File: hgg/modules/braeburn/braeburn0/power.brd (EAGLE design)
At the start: 104.4 x 75 mm, 69 parts, among them IC1 LM324D, IC4 ATMEGA48/88/168-AU, IC5 LTC485S, Q1 20Mhz

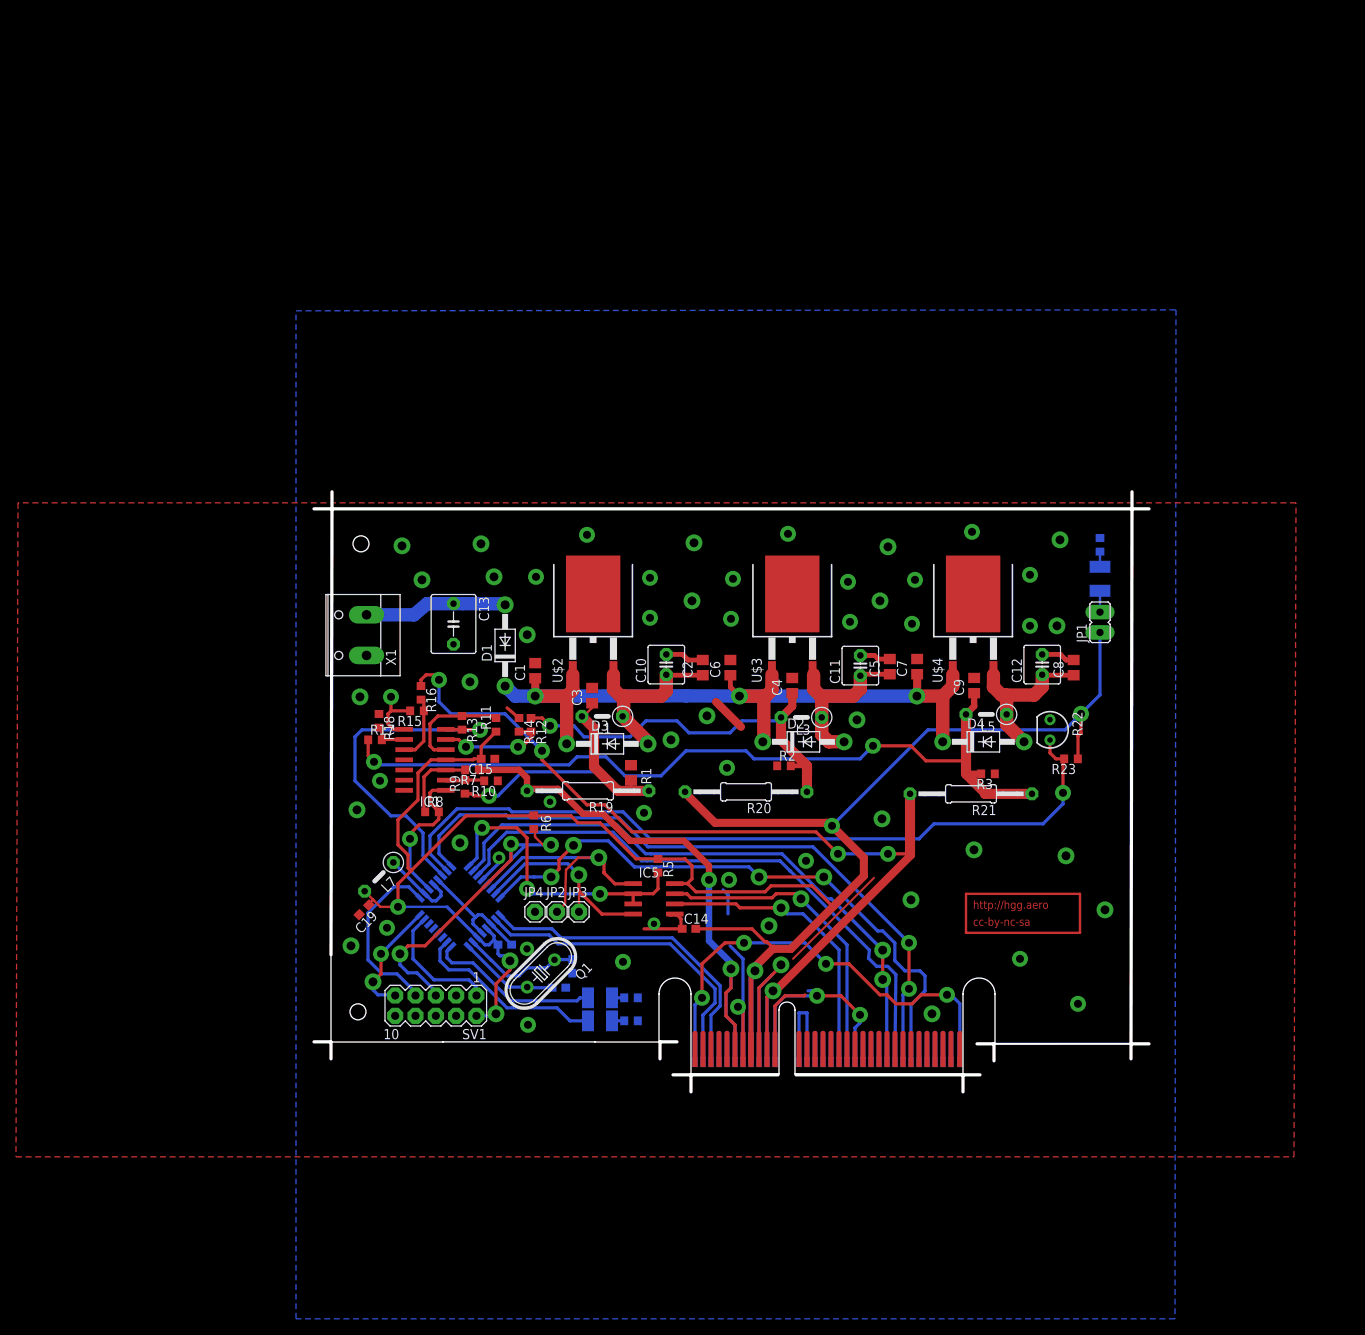
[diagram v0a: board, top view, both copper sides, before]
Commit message: updates versoin of braeburn
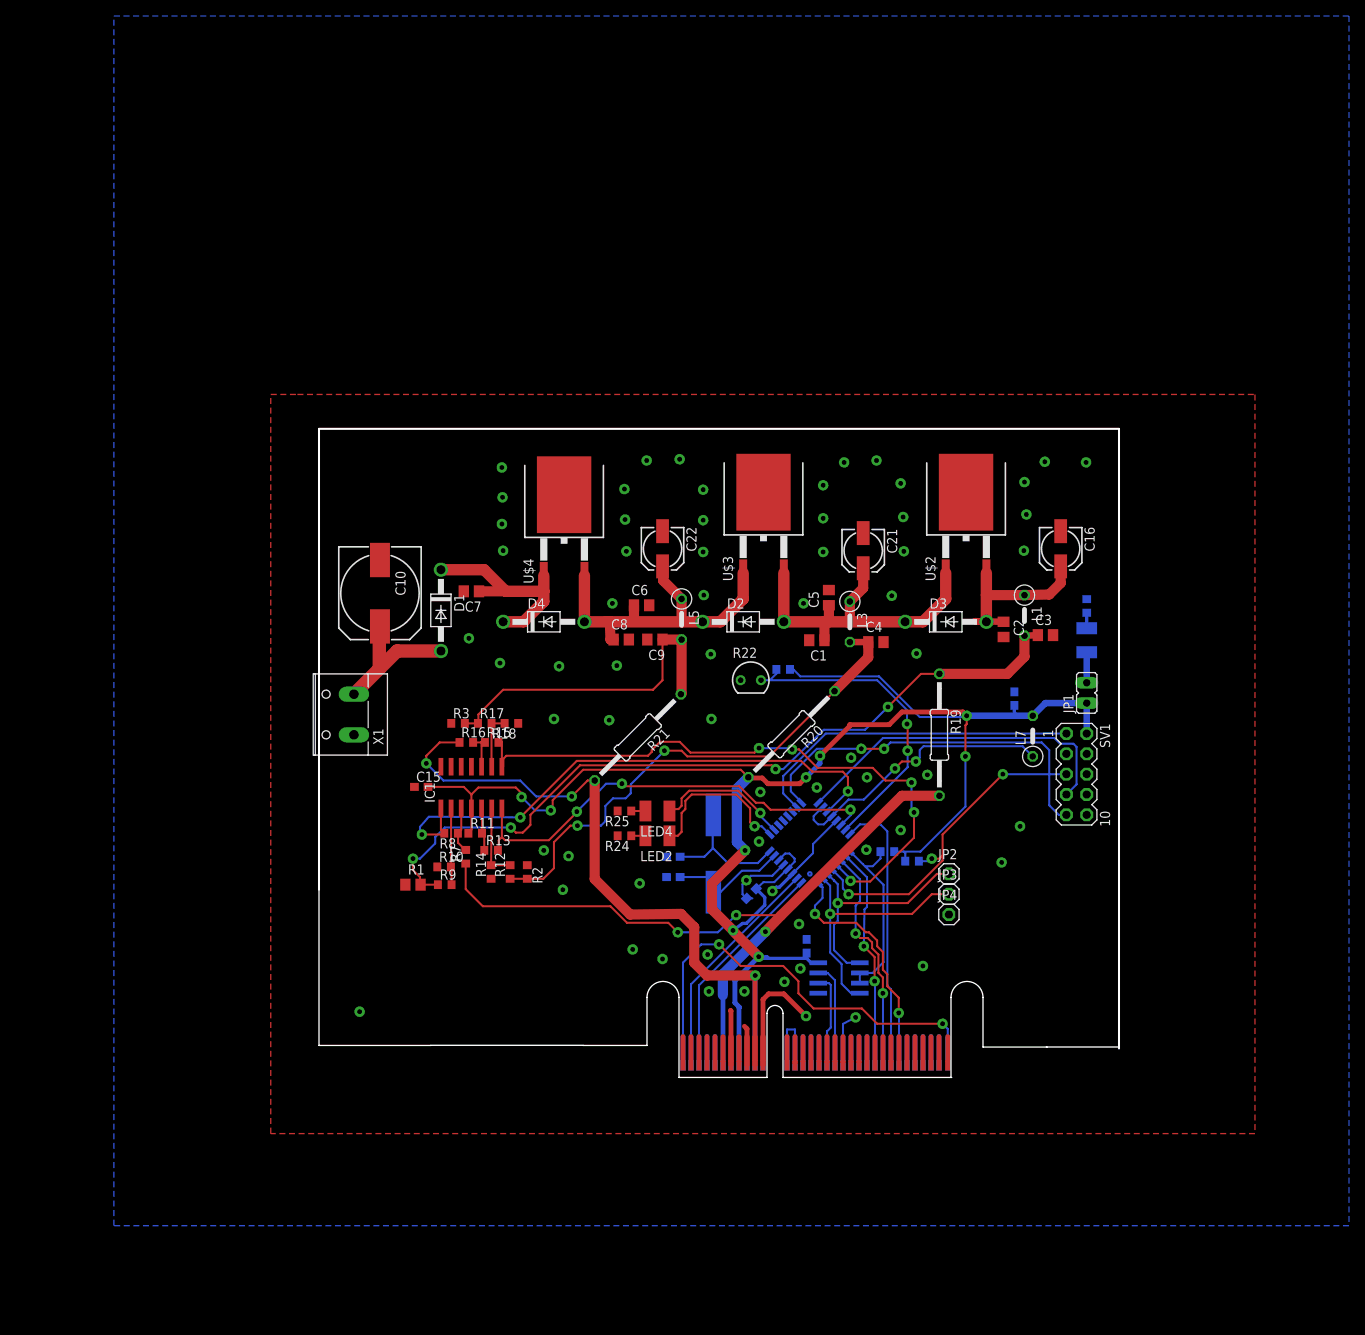
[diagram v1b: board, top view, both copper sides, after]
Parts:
- removed C11, C12: (no value), rcl:C025-050X050
- removed C13: 2000u, resistor:C050-055X075
- added C16, C21, C22: (no value), rcl:153CLV-0505
- C10: device rcl:C025-050X050 -> rcl:150CLZ-1010
- Q1: device crystal:HC49U-V -> crystal:HC49UP
- moved C19 85.5 mm to (86.9, 46.3), flipped to the bottom, turned to 90 degrees
- moved SV1 85.2 mm to (94.7, 36.8), turned to 270 degrees
- moved L7 83.6 mm to (89.2, 41.6), turned to 90 degrees
- moved R3 66.5 mm to (17.4, 43.2), turned to 0 degrees
- moved C3 57.2 mm to (90.8, 54.2), turned to 0 degrees
- moved D4 57.0 mm to (28.1, 55.9)
- moved C8 56.7 mm to (37.8, 53.7), turned to 0 degrees
- moved C7 56.5 mm to (19.1, 59.7), turned to 180 degrees
- moved L1 54.3 mm to (88.2, 56.7), turned to 270 degrees
- moved U$4 52.6 mm to (30.6, 68.3)
- moved JP4 51.7 mm to (78.7, 19.3)
- moved JP2 49.2 mm to (78.7, 24.4)
- moved U$2 48.3 mm to (80.9, 68.6)
- moved R6 47.5 mm to (74.1, 26.0), flipped to the bottom, turned to 180 degrees
- moved JP3 46.3 mm to (78.7, 21.8)
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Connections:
- removed net N$1: C1.1, C6.1, C7.1, D1.C, D2.C, D3.C, D4.C, U$2.1, U$3.1, U$4.1
- removed net N$3: C12.1, C8.1, D4.A, L5.1, U$4.2
- removed net N$4: C11.1, C5.1, D2.A, L3.1, U$3.2
- new net 12VOUT: C22.+, C6.1, C8.1, D2.C, D4.A, L5.1, U$3.1, U$4.2
- new net 5VOUT: C1.1, C21.+, C5.1, D2.A, D3.C, L3.1, U$2.1, U$3.2
- new net N$11: C7.1, D1.C, D4.C, U$4.1
- net 3V3: no longer U$1.B06(+3V3)
- net GND: now also C10.-, C16.-, C21.-, C22.-; no longer C10.2, C11.2, C12.2, C13.2, U$1.A07(GND), U$1.A09(GND), U$1.A11(GND)
- net N$12: now also C10.+; no longer C13.1
- net N$5: now also C16.+; no longer C10.1
- net VCC: no longer U$1.B08(+5V)
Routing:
- net N$1: track 97.8 -> 0.00 mm, vias 3 -> 0
- net GND: track 153.0 -> 55.8 mm, vias 57 -> 66
- net MEASURE12V: track 13.0 -> 79.2 mm, vias 2 -> 5
- net 12VIN: track 103.6 -> 41.9 mm, vias 2 -> 0
- net TEMP1: track 98.7 -> 39.7 mm, vias 1 -> 2
- net 3V3IN: track 45.5 -> 99.1 mm, vias 1 -> 4
- net MEASURE3V3: track 18.1 -> 70.4 mm, vias 1 -> 3
- net N$6: track 86.1 -> 35.0 mm, vias 2 -> 0
- net 12VOUT: track 0.00 -> 49.5 mm
- net N$25: track 75.5 -> 28.0 mm
- net VCC: track 269.3 -> 222.1 mm, vias 6 -> 9
- net N$20: track 76.6 -> 30.4 mm, vias 4 -> 2
- net N$24: track 74.6 -> 28.8 mm, vias 0 -> 2
- net 5VOUT: track 0.00 -> 42.7 mm
- net N$31: track 38.2 -> 0.00 mm
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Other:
- board size 104.4 x 75 mm -> 100 x 77.5 mm
- board text removed: "12V"
- board text removed: "3v3"
- board text removed: "5V"
- board text removed: "cc-by-nc-sa"
- board text removed: "http://hgg.aero"
